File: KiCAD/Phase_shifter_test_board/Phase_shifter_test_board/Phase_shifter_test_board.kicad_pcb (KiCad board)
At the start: 2 copper layers, 30.5 x 25.2 mm, 7 parts, among them J3 Conn_01x10_Pin

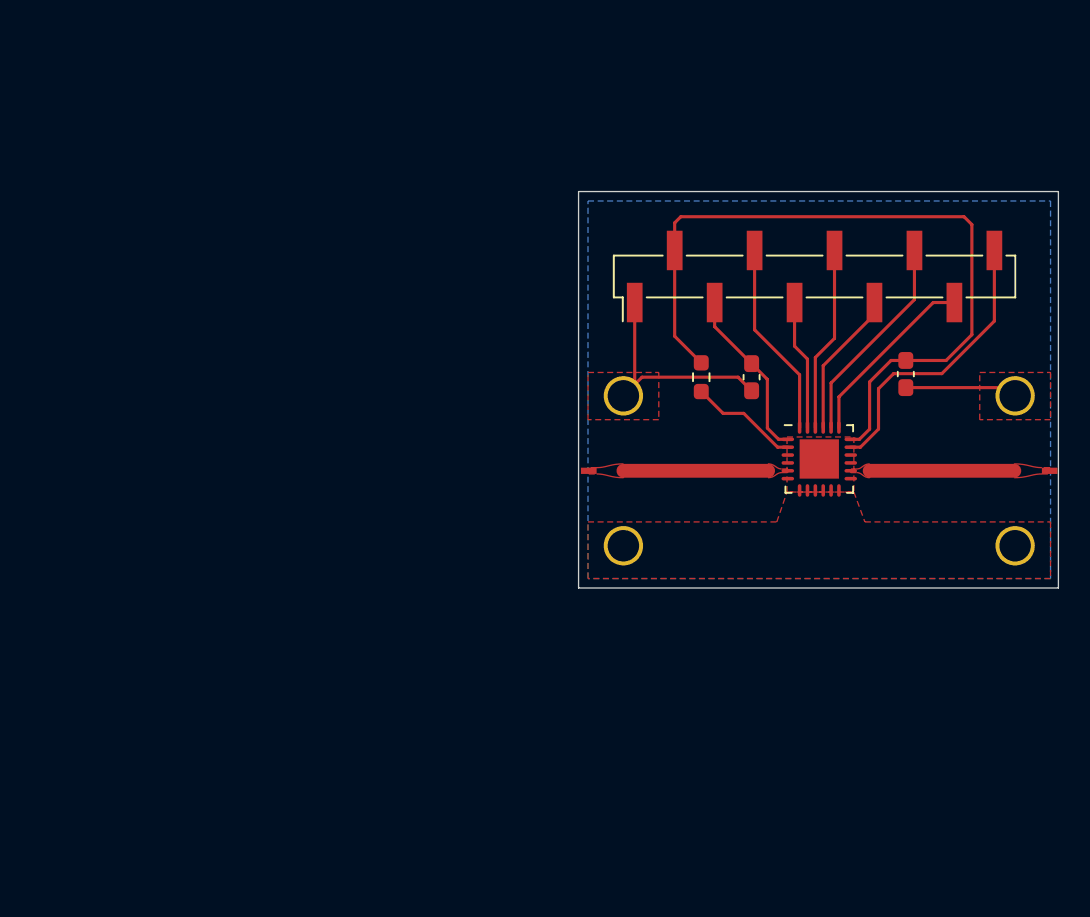
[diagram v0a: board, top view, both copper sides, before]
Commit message: phase shifter
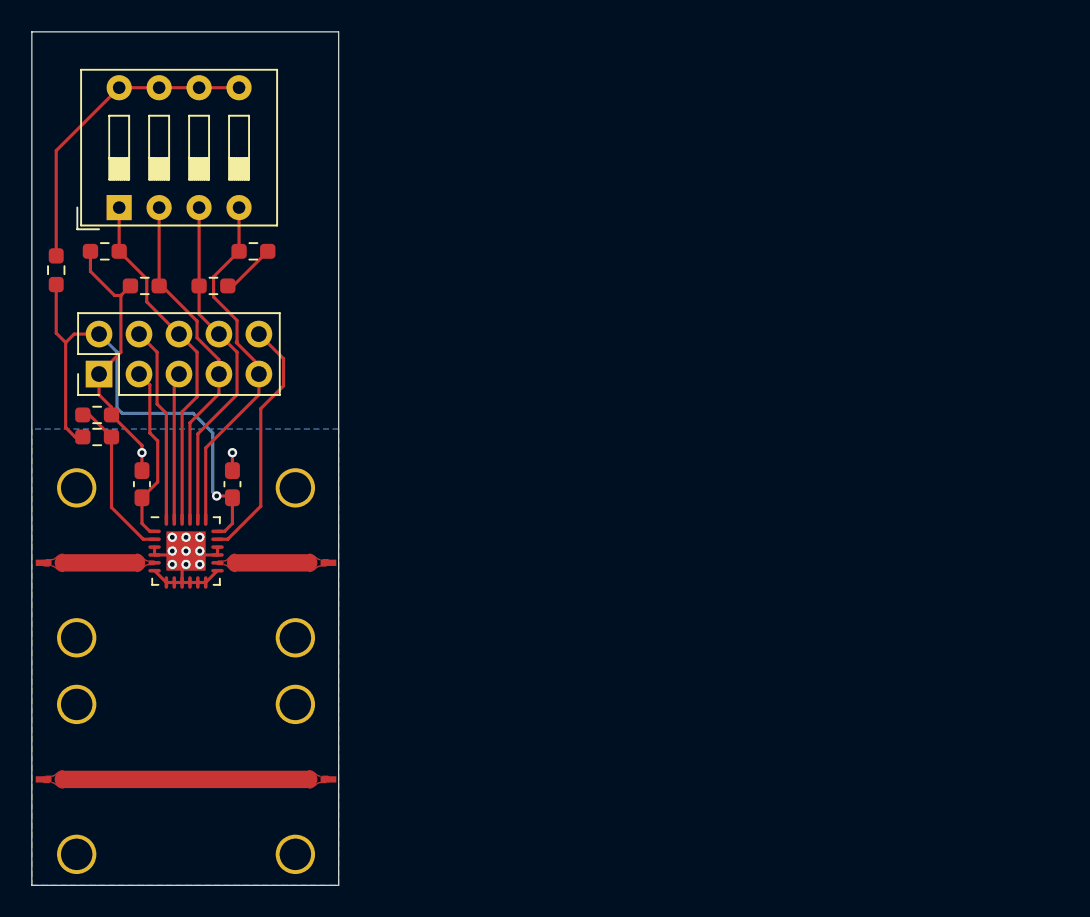
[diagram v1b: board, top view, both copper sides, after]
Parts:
- added J4: ~, Phase_shifter:Conn, F.Cu at (117.0, 114.8)
- added J5: Conn_02x05_Odd_Even, Connector_PinHeader_2.54mm:PinHeader_2x05_P2.54mm_Vertical, F.Cu at (104.5, 89.0)
- added R2: R, Resistor_SMD:R_0603_1608Metric_Pad0.98x0.95mm_HandSolder, F.Cu at (104.9, 81.2)
- added R3: R, Resistor_SMD:R_0603_1608Metric_Pad0.98x0.95mm_HandSolder, F.Cu at (107.4, 83.4)
- added R4: R, Resistor_SMD:R_0603_1608Metric_Pad0.98x0.95mm_HandSolder, F.Cu at (111.8, 83.4)
- added R5: R, Resistor_SMD:R_0603_1608Metric_Pad0.98x0.95mm_HandSolder, F.Cu at (114.3, 81.2)
- added R6: R, Resistor_SMD:R_0603_1608Metric_Pad0.98x0.95mm_HandSolder, F.Cu at (101.8, 82.4)
- added R7: R, Resistor_SMD:R_0603_1608Metric_Pad0.98x0.95mm_HandSolder, F.Cu at (104.4, 91.6)
- added SW1: SW_DIP_x04, Button_Switch_THT:SW_DIP_SPSTx04_Slide_9.78x12.34mm_W7.62mm_P2.54mm, F.Cu at (105.8, 78.4)
- J3: value Conn_01x10_Pin -> ~; footprint Connector_PinHeader_2.54mm:PinHeader_1x10_P2.54mm_Vertical_SMD_Pin1Left -> Phase_shifter:Conn
- moved J3 56.8 mm to (103.1, 114.8)
- moved J2 46.1 mm to (117.0, 101.0)
- moved C2 43.4 mm to (113.0, 96.0), turned to 90 degrees
- moved U1 40.7 mm to (110.0, 100.2)
- moved C1 39.3 mm to (107.2, 96.0), turned to 90 degrees
- moved R1 38.6 mm to (104.4, 93.0), turned to 0 degrees
- moved J1 35.2 mm to (103.1, 101.0)
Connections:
- J3 pad 1: GND -> /RF REF
- J3 pad 2: VCC -> GND
- U1 pad 22: /LE -> /LE / D3
- U1 pad 23: /CLK -> /CLK / D2
- U1 pad 24: /SER IN -> /SER IN / D1
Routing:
- net /LE / D3: track 0.00 -> 22.5 mm
- net Net-(R6-Pad1): track 0.00 -> 20.0 mm
- net /RF REF: track 0.00 -> 15.6 mm
- net VCC: track 48.1 -> 32.9 mm, vias 0 -> 1
- net /D4: track 9.30 -> 22.3 mm
- net /SER IN / D1: track 0.00 -> 12.5 mm
- net /SER IN: track 12.4 -> 0.00 mm
- net /LE: track 11.8 -> 0.00 mm
- net /D6: track 11.8 -> 23.1 mm
- net /CLK / D2: track 0.00 -> 9.37 mm
- net GND: track 22.4 -> 31.5 mm, vias 0 -> 11
- net /D5: track 13.5 -> 21.9 mm
- net /CLK: track 8.28 -> 0.00 mm
- net /RF IN: track 9.20 -> 4.65 mm
- net /RF OUT: track 9.20 -> 4.65 mm
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- added copper zone on F.Cu, net /RF REF
- removed copper zone on F.Cu, net GND
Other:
- board size 30.5 x 25.2 mm -> 19.5 x 54.2 mm
